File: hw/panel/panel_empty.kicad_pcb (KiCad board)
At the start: 4 copper layers, 158 x 89 mm, 13 parts

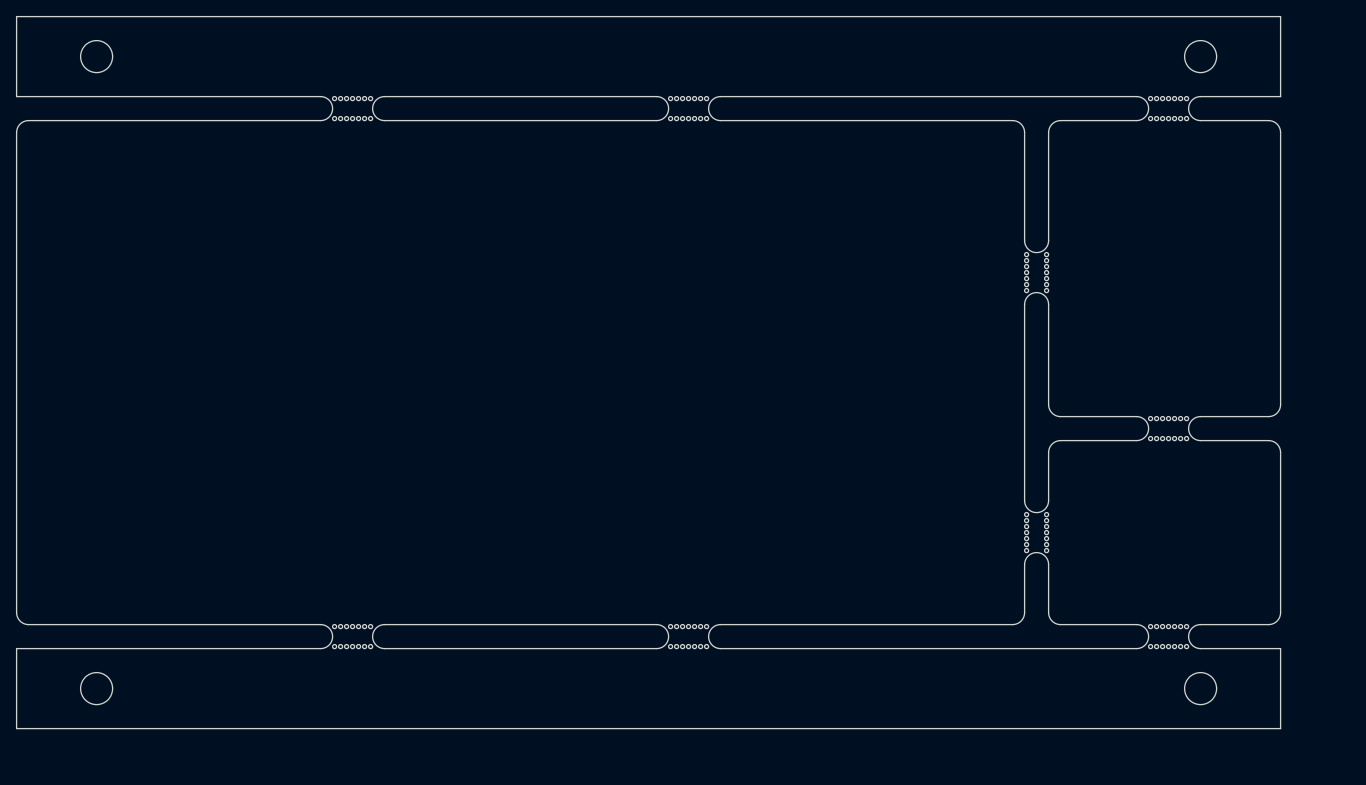
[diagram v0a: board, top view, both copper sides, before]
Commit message: temp commit for merge
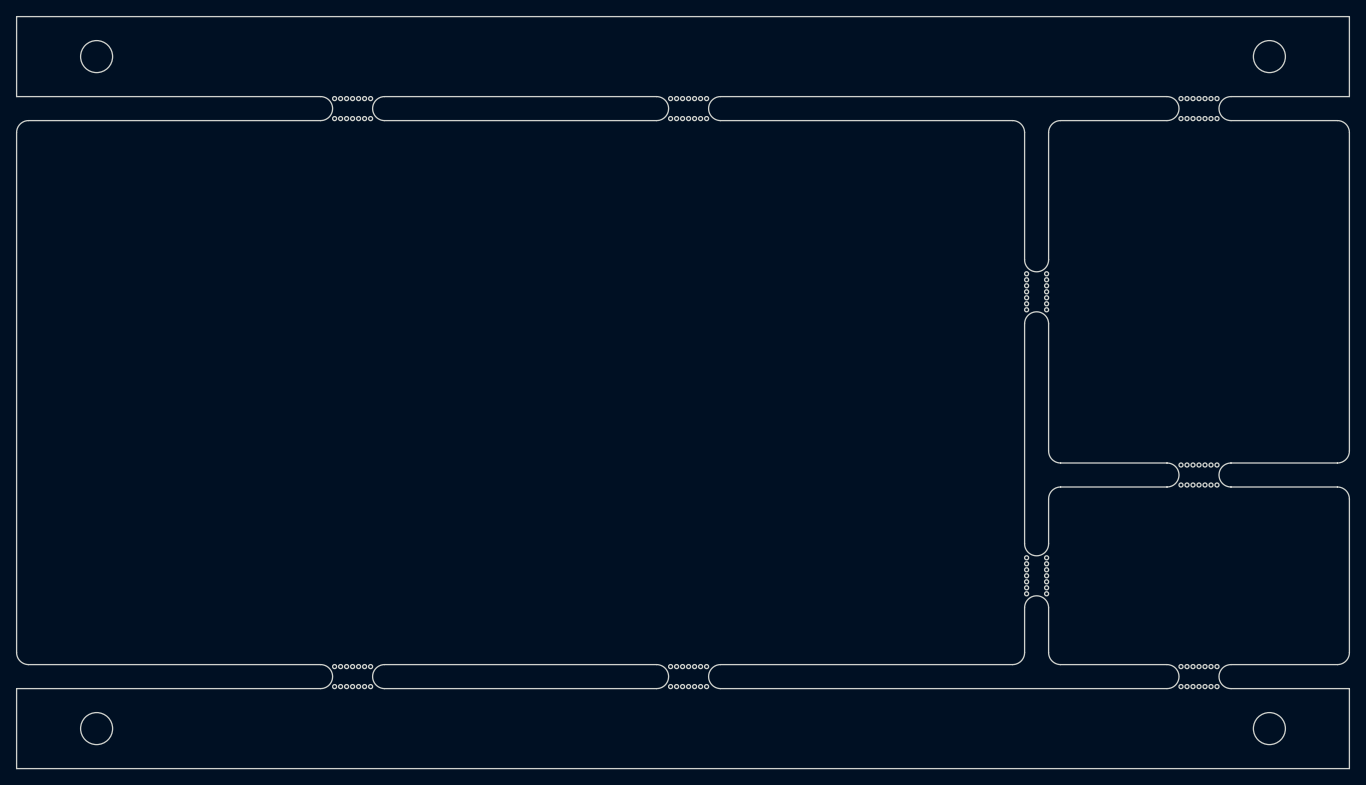
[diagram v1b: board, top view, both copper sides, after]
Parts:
- removed the REF** at (183.5, 114.5)
- removed the REF** at (183.5, 82.0)
- removed the REF** at (98.0, 127.5)
- removed the REF** at (140.0, 127.5)
- removed the REF** at (200.0, 127.5)
- removed the REF** at (200.0, 101.5)
- removed the REF** at (200.0, 61.5)
- added REF**: mouse-bite-3mm-slot, panelization:mouse-bite-3mm-slot, F.Cu at (183.5, 119.9)
- added REF**: mouse-bite-3mm-slot, panelization:mouse-bite-3mm-slot, F.Cu at (183.5, 84.4)
- added REF**: mouse-bite-3mm-slot, panelization:mouse-bite-3mm-slot, F.Cu at (98.0, 132.5)
- added REF**: mouse-bite-3mm-slot, panelization:mouse-bite-3mm-slot, F.Cu at (140.0, 132.5)
- added REF**: mouse-bite-3mm-slot, panelization:mouse-bite-3mm-slot, F.Cu at (203.8, 132.5)
- added REF**: mouse-bite-3mm-slot, panelization:mouse-bite-3mm-slot, F.Cu at (203.8, 107.3)
- added REF**: mouse-bite-3mm-slot, panelization:mouse-bite-3mm-slot, F.Cu at (203.8, 61.5)
- moved REF** 9.95 mm to (212.6, 139.0)
- moved REF** 8.60 mm to (212.6, 55.0)
- moved REF** 5.00 mm to (66.0, 139.0)
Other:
- board size 158 x 89 mm -> 166.6 x 94 mm
